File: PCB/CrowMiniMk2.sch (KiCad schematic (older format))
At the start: 21 parts, among them J1 AVR-ISP-6, SW1 SW_Push, U1 ATmega32U4-AU, U2 PRTR5V0U2X, X1 XTAL

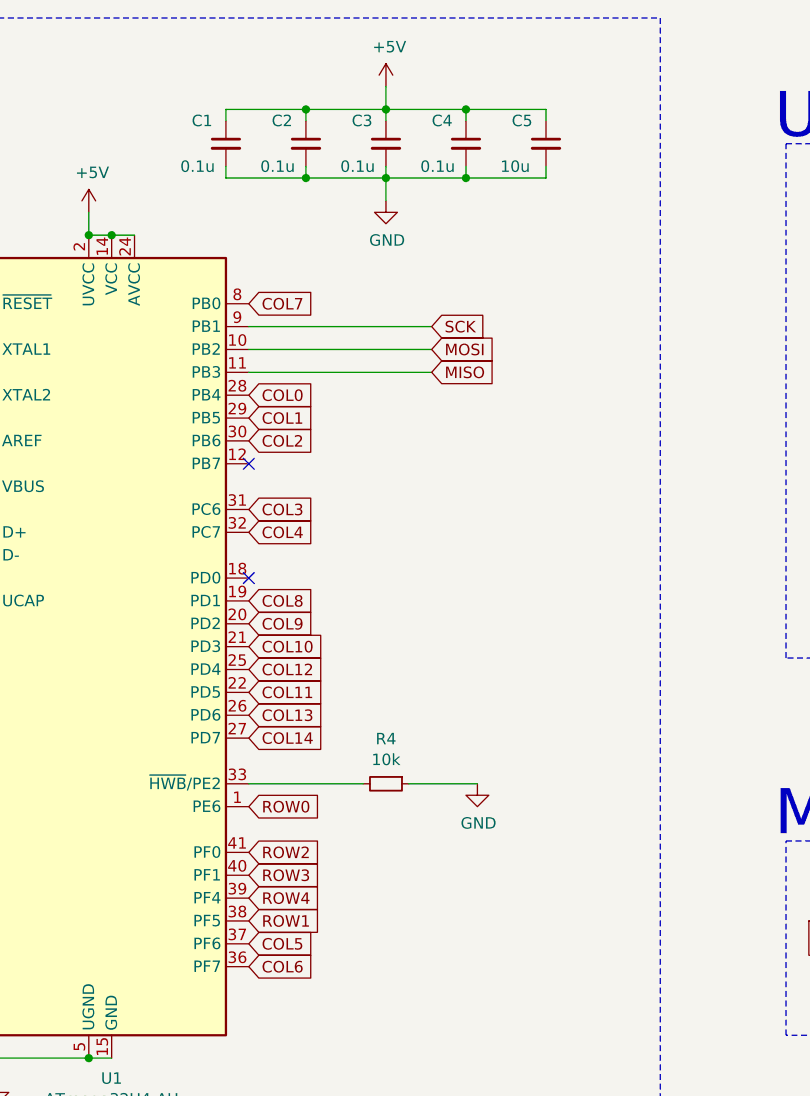
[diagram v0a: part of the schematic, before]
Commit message: Routing 99%
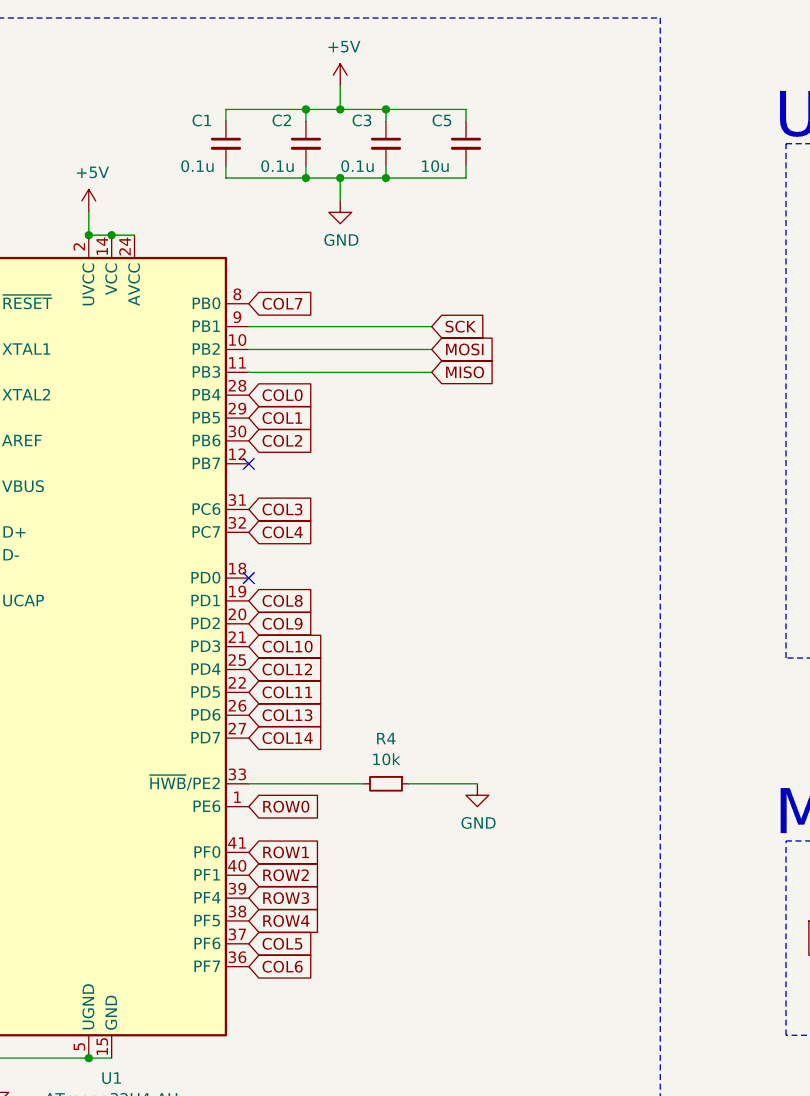
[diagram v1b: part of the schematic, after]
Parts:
- removed C4: 0.1u, Capacitor_SMD:C_0805_2012Metric_Pad1.15x1.40mm_HandSolder, symbol Device:C_Small
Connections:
- net ROW1: now also U1.41 (PF0); no longer U1.38 (PF5)
- net ROW2: now also U1.40 (PF1); no longer U1.41 (PF0)
- net ROW3: now also U1.39 (PF4); no longer U1.40 (PF1)
- net ROW4: now also U1.38 (PF5); no longer U1.39 (PF4)
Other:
- moved on the sheet: C5
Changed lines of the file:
@@
 EESchema Schematic File Version 4
+LIBS:CrowMiniMk2-cache
 EELAYER 30 0
 EELAYER END
@@
 Wire Wire Line
 	3400 1000 3750 1000
-Wire Wire Line
-	4800 1000 4800 1050
-Wire Wire Line
-	4450 1000 4450 1050
-Connection ~ 4450 1000
-Wire Wire Line
-	4450 1000 4800 1000
 Connection ~ 4100 1000
-Wire Wire Line
-	4100 1000 4450 1000
 Wire Wire Line
 	3750 1050 3750 1000
 Connection ~ 3750 1000
 Wire Wire Line
-	3750 1000 4100 1000
+	3750 1000 3900 1000
 Wire Wire Line
 	3400 1250 3400 1300
 Wire Wire Line
 	3400 1300 3750 1300
-Wire Wire Line
-	4800 1300 4800 1250
-Wire Wire Line
-	4450 1250 4450 1300
-Connection ~ 4450 1300
-Wire Wire Line
-	4450 1300 4800 1300
 Connection ~ 4100 1300
-Wire Wire Line
-	4100 1300 4450 1300
 Wire Wire Line
 	3750 1250 3750 1300
 Connection ~ 3750 1300
 Wire Wire Line
-	3750 1300 4100 1300
-Wire Wire Line
-	4100 1000 4100 900
-Wire Wire Line
-	4100 1300 4100 1400
+	3750 1300 3900 1300
+Wire Wire Line
+	3900 1000 3900 900
+Wire Wire Line
+	3900 1300 3900 1400
 $Comp
 L power:GND #PWR0106
 U 1 1 61532139
-P 4100 1400
-F 0 "#PWR0106" H 4100 1150 50  0001 C CNN
-F 1 "GND" H 4105 1227 50  0000 C CNN
-F 2 "" H 4100 1400 50  0001 C CNN
-F 3 "" H 4100 1400 50  0001 C CNN
-	1    4100 1400
+P 3900 1400
+F 0 "#PWR0106" H 3900 1150 50  0001 C CNN
+F 1 "GND" H 3905 1227 50  0000 C CNN
+F 2 "" H 3900 1400 50  0001 C CNN
+F 3 "" H 3900 1400 50  0001 C CNN
+	1    3900 1400
 	1    0    0    -1
 $EndComp
@@
 L power:+5V #PWR0107
 U 1 1 61532DEE
-P 4100 900
-F 0 "#PWR0107" H 4100 750 50  0001 C CNN
-F 1 "+5V" H 4115 1073 50  0000 C CNN
-F 2 "" H 4100 900 50  0001 C CNN
-F 3 "" H 4100 900 50  0001 C CNN
-	1    4100 900
+P 3900 900
+F 0 "#PWR0107" H 3900 750 50  0001 C CNN
+F 1 "+5V" H 3915 1073 50  0000 C CNN
+F 2 "" H 3900 900 50  0001 C CNN
+F 3 "" H 3900 900 50  0001 C CNN
+	1    3900 900
 	1    0    0    -1
 $EndComp
@@
 Text GLabel 3500 4050 2    50   Input ~ 0
 ROW0
+Text GLabel 3500 4350 2    50   Input ~ 0
+ROW2
+Text GLabel 3500 4450 2    50   Input ~ 0
+ROW3
+Text GLabel 3500 4550 2    50   Input ~ 0
+ROW4
 Text GLabel 3500 4250 2    50   Input ~ 0
-ROW2
-Text GLabel 3500 4350 2    50   Input ~ 0
-ROW3
-Text GLabel 3500 4450 2    50   Input ~ 0
-ROW4
-Text GLabel 3500 4550 2    50   Input ~ 0
 ROW1
 Text GLabel 3500 4650 2    50   Input ~ 0
@@
 L Device:C_Small C5
 U 1 1 615241AC
-P 4800 1150
-F 0 "C5" H 4650 1250 50  0000 L CNN
-F 1 "10u" H 4600 1050 50  0000 L CNN
-F 2 "Capacitor_SMD:C_0805_2012Metric_Pad1.15x1.40mm_HandSolder" H 4800 1150 50  0001 C CNN
-F 3 "~" H 4800 1150 50  0001 C CNN
-	1    4800 1150
-	1    0    0    -1
-$EndComp
-$Comp
-L Device:C_Small C4
-U 1 1 61521C69
 P 4450 1150
-F 0 "C4" H 4300 1250 50  0000 L CNN
-F 1 "0.1u" H 4250 1050 50  0000 L CNN
+F 0 "C5" H 4300 1250 50  0000 L CNN
+F 1 "10u" H 4250 1050 50  0000 L CNN
 F 2 "Capacitor_SMD:C_0805_2012Metric_Pad1.15x1.40mm_HandSolder" H 4450 1150 50  0001 C CNN
 F 3 "~" H 4450 1150 50  0001 C CNN
@@
 Wire Wire Line
 	4100 1050 4100 1000
+Text GLabel 7800 2200 1    50   Input ~ 0
+DN
+Text GLabel 7800 2300 3    50   Input ~ 0
+DP
 $Comp
 L Device:C_Small C3
@@
 	1    0    0    -1
 $EndComp
-Text GLabel 7800 2200 1    50   Input ~ 0
-DN
-Text GLabel 7800 2300 3    50   Input ~ 0
-DP
+Wire Wire Line
+	4100 1000 4450 1000
+Wire Wire Line
+	4450 1000 4450 1050
+Wire Wire Line
+	4450 1250 4450 1300
+Wire Wire Line
+	4450 1300 4100 1300
+Connection ~ 3900 1000
+Wire Wire Line
+	3900 1000 4100 1000
+Connection ~ 3900 1300
+Wire Wire Line
+	3900 1300 4100 1300
 $EndSCHEMATC

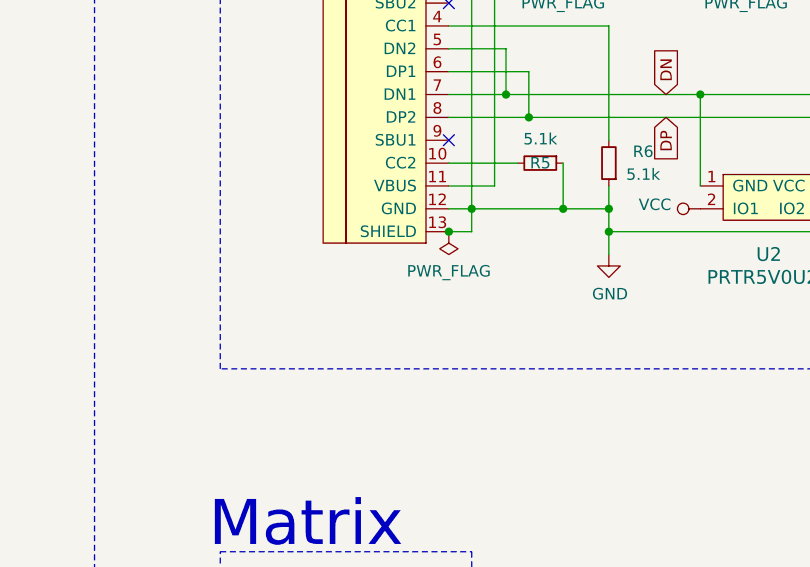
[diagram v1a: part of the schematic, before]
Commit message: Pre Logo add
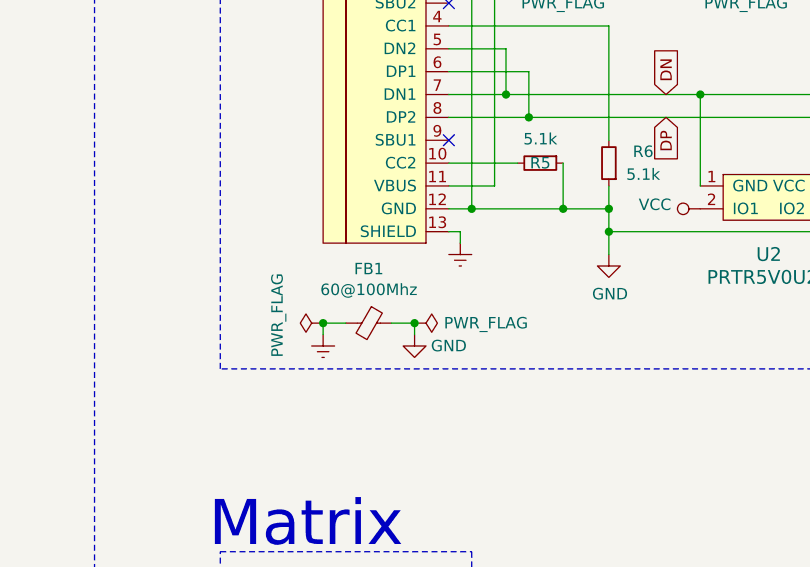
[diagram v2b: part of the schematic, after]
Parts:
- added FB1: 60@100Mhz, Inductor_SMD:L_0805_2012Metric_Pad1.15x1.40mm_HandSolder, symbol Device:Ferrite_Bead_Small
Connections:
- net GND: now also FB1.1; no longer USB1.13 (SHIELD)
- new net Earth: FB1.2, USB1.13 (SHIELD)
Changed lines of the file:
@@
 D-
-Wire Wire Line
-	6850 2800 6950 2800
-Wire Wire Line
-	6950 2800 6950 2700
 Wire Wire Line
 	6950 1600 6850 1600
@@
 Text Notes 5800 1150 0    197  ~ 0
 USB Type C
-$Comp
-L power:PWR_FLAG #FLG0101
-U 1 1 619CFD75
-P 6850 2800
-F 0 "#FLG0101" H 6850 2875 50  0001 C CNN
-F 1 "PWR_FLAG" H 6850 2973 50  0000 C CNN
-F 2 "" H 6850 2800 50  0001 C CNN
-F 3 "~" H 6850 2800 50  0001 C CNN
-	1    6850 2800
-	-1   0    0    1
-$EndComp
-Connection ~ 6850 2800
 Connection ~ 7200 1700
 Wire Wire Line
@@
 Wire Wire Line
 	3900 1300 4100 1300
+Wire Wire Line
+	6850 2800 6900 2800
+Wire Wire Line
+	6900 2800 6900 2850
+$Comp
+L power:Earth #PWR0117
+U 1 1 61581AB9
+P 6900 2850
+F 0 "#PWR0117" H 6900 2600 50  0001 C CNN
+F 1 "Earth" H 6900 2700 50  0001 C CNN
+F 2 "" H 6900 2850 50  0001 C CNN
+F 3 "~" H 6900 2850 50  0001 C CNN
+	1    6900 2850
+	1    0    0    -1
+$EndComp
+$Comp
+L Device:Ferrite_Bead_Small FB1
+U 1 1 61585633
+P 6500 3200
+F 0 "FB1" V 6263 3200 50  0000 C CNN
+F 1 "60@100Mhz" V 6354 3200 50  0000 C CNN
+F 2 "Inductor_SMD:L_0805_2012Metric_Pad1.15x1.40mm_HandSolder" V 6430 3200 50  0001 C CNN
+F 3 "~" H 6500 3200 50  0001 C CNN
+	1    6500 3200
+	0    1    1    0
+$EndComp
+Wire Wire Line
+	6600 3200 6700 3200
+Wire Wire Line
+	6700 3200 6700 3250
+Wire Wire Line
+	6400 3200 6300 3200
+Wire Wire Line
+	6300 3200 6300 3250
+$Comp
+L power:Earth #PWR0118
+U 1 1 6158C020
+P 6300 3250
+F 0 "#PWR0118" H 6300 3000 50  0001 C CNN
+F 1 "Earth" H 6300 3100 50  0001 C CNN
+F 2 "" H 6300 3250 50  0001 C CNN
+F 3 "~" H 6300 3250 50  0001 C CNN
+	1    6300 3250
+	1    0    0    -1
+$EndComp
+$Comp
+L power:GND #PWR0119
+U 1 1 6158D048
+P 6700 3250
+F 0 "#PWR0119" H 6700 3000 50  0001 C CNN
+F 1 "GND" H 6850 3200 50  0000 C CNN
+F 2 "" H 6700 3250 50  0001 C CNN
+F 3 "" H 6700 3250 50  0001 C CNN
+	1    6700 3250
+	1    0    0    -1
+$EndComp
+$Comp
+L power:PWR_FLAG #FLG0101
+U 1 1 6158E0C6
+P 6300 3200
+F 0 "#FLG0101" H 6300 3275 50  0001 C CNN
+F 1 "PWR_FLAG" H 6150 3400 50  0000 L CNN
+F 2 "" H 6300 3200 50  0001 C CNN
+F 3 "~" H 6300 3200 50  0001 C CNN
+	1    6300 3200
+	0    -1   -1   0
+$EndComp
+Connection ~ 6300 3200
+$Comp
+L power:PWR_FLAG #FLG0104
+U 1 1 6158E526
+P 6700 3200
+F 0 "#FLG0104" H 6700 3275 50  0001 C CNN
+F 1 "PWR_FLAG" V 6700 3328 50  0000 L CNN
+F 2 "" H 6700 3200 50  0001 C CNN
+F 3 "~" H 6700 3200 50  0001 C CNN
+	1    6700 3200
+	0    1    1    0
+$EndComp
+Connection ~ 6700 3200
 $EndSCHEMATC
